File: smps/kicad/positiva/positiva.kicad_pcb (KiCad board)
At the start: 2 copper layers, 124.5 x 72.4 mm, 13 parts, among them J1 Conn_01x01_Female, J2 Conn_01x01_Female, J3 Conn_01x01_Female, J4 Conn_01x01_Female, U1 LM2576T-ADJ

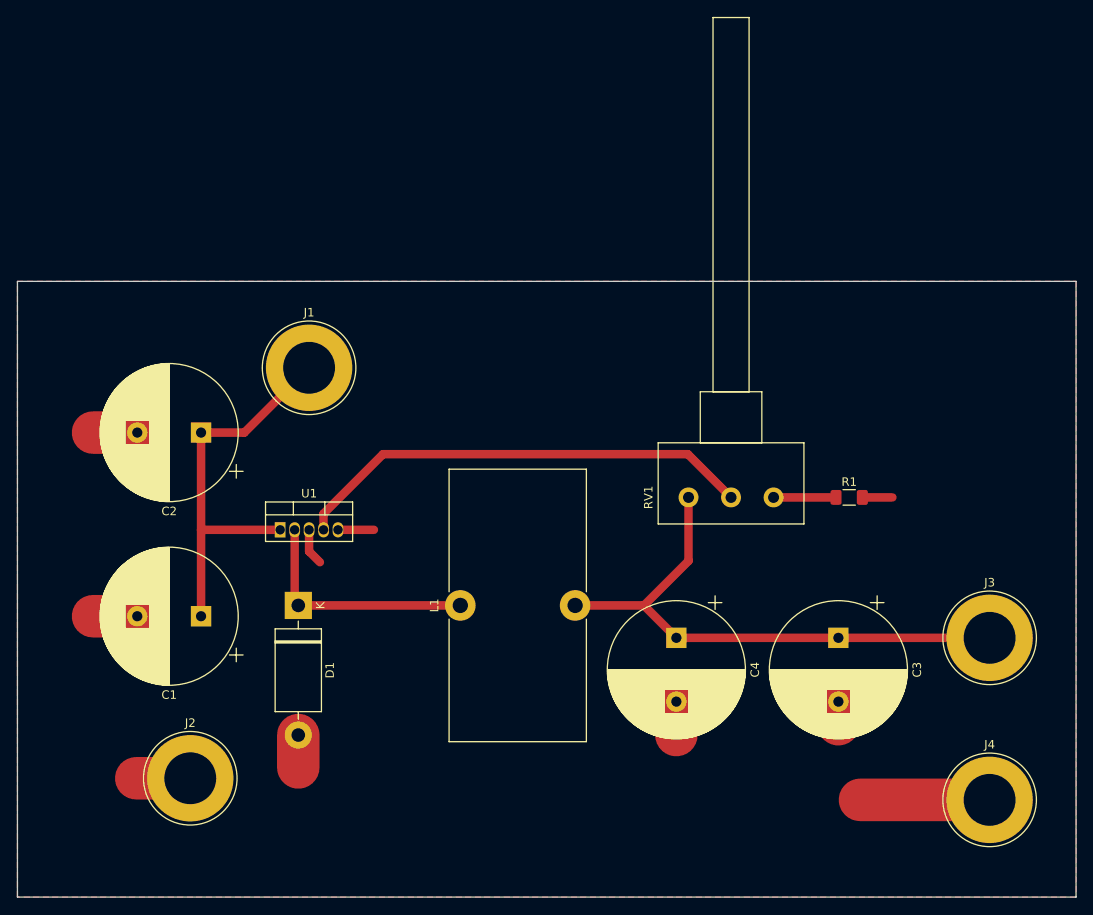
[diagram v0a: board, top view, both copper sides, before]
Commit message: varias cosas, layouts de fuentes terminados, calculo de componentes completo
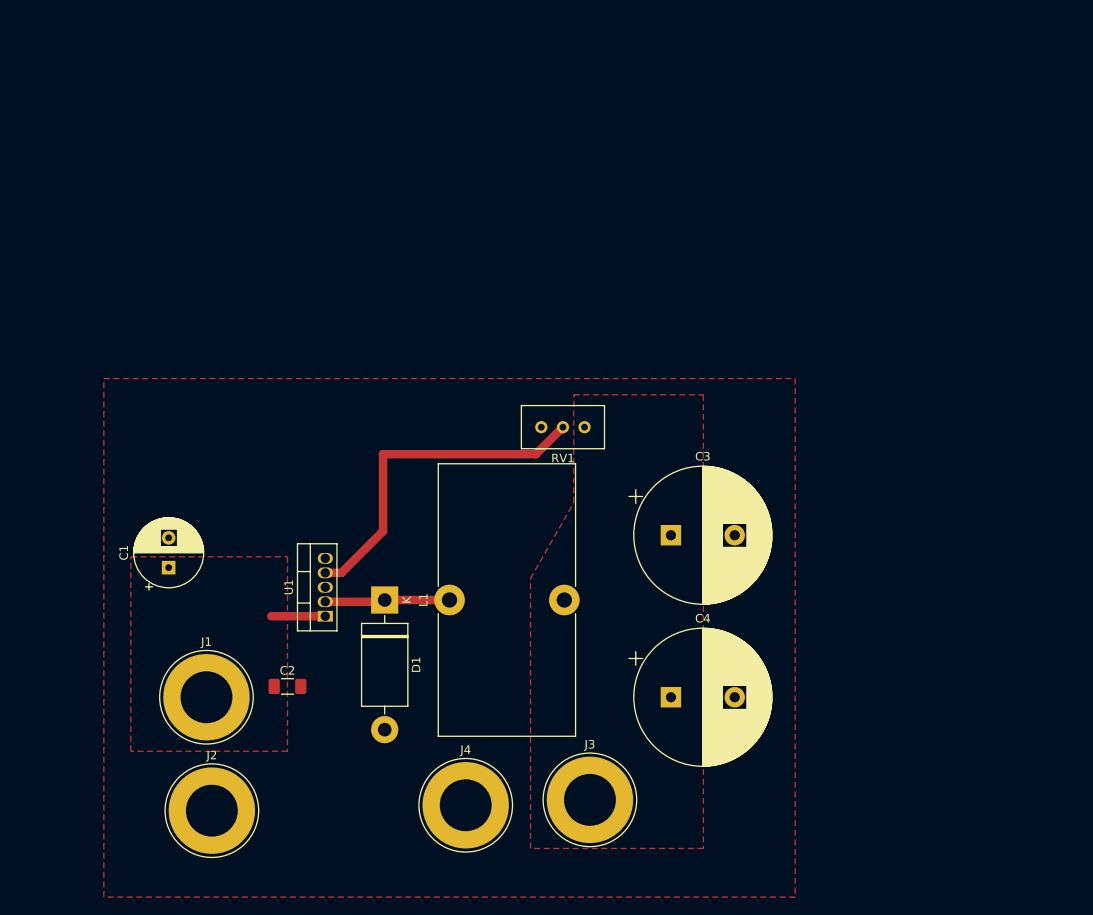
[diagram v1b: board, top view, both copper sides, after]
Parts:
- removed R1: 1.2k, Resistor_SMD:R_1206_3216Metric_Pad1.30x1.75mm_HandSolder
- C1: footprint Capacitor_THT:CP_Radial_D16.0mm_P7.50mm -> Capacitor_THT:CP_Radial_D8.0mm_P3.50mm
- C2: value 100u -> 0.22u; footprint Capacitor_THT:CP_Radial_D16.0mm_P7.50mm -> Capacitor_SMD:C_1206_3216Metric_Pad1.33x1.80mm_HandSolder
- RV1: value 50k -> 100k; footprint Potentiometer_THT:Potentiometer_Omeg_PC16BU_Horizontal -> Potentiometer_THT:Potentiometer_Bourns_3296W_Vertical
- moved J4 61.6 mm to (155.6, 153.0)
- moved J3 50.7 mm to (170.2, 152.4)
- moved J1 40.6 mm to (125.1, 140.3)
- moved C2 31.5 mm to (134.6, 139.1), turned to 0 degrees
- moved RV1 28.5 mm to (164.5, 108.6), turned to 180 degrees
- moved C3 23.1 mm to (179.7, 121.3), turned to 0 degrees
- moved U1 11.5 mm to (139.1, 130.8), turned to 90 degrees
- moved D1 10.2 mm to (146.1, 128.9)
- moved C4 7.01 mm to (179.7, 140.3), turned to 0 degrees
- moved C1 6.87 mm to (120.7, 125.1), turned to 90 degrees
- moved J2 4.58 mm to (125.7, 153.7)
- moved L1 1.42 mm to (153.7, 128.9)
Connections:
- RV1 pad 1: Net-(R1-Pad1) -> GND
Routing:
- net /VoutDC: track 65.2 -> 0.00 mm
- net GND: track 54.5 -> 0.00 mm
- net /Vin: track 46.7 -> 6.35 mm
- net /Vfb: track 54.8 -> 40.3 mm
- net /VoutSW: track 28.7 -> 14.7 mm
- net Net-(R1-Pad1): track 7.34 -> 0.00 mm
- added copper zone on F.Cu, net /Vin
- added copper zone on F.Cu, net /VoutDC
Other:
- board outline removed

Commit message: last minute commit
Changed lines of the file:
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@@
   (general
     (thickness 1.6)
-    (drawings 2)
+    (drawings 0)
     (tracks 9)
     (zones 0)
@@
   )
   (setup
-    (last_trace_width 1)
+    (last_trace_width 0.3048)
     (user_trace_width 1)
     (user_trace_width 5)
@@
     (visible_elements FFFFFF7F)
     (pcbplotparams
-      (layerselection 0x010fc_ffffffff)
+      (layerselection 0x01088_7fffffff)
       (usegerberextensions false)
       (usegerberattributes true)
@@
       (outputformat 1)
       (mirror false)
-      (drillshape 1)
+      (drillshape 0)
       (scaleselection 1)
       (outputdirectory ""))
@@
       (effects (font (size 1 1) (thickness 0.15)))
     )
-    (fp_text user %R (at 0 0) (layer F.Fab)
-      (effects (font (size 0.8 0.8) (thickness 0.12)))
-    )
     (fp_line (start -1.6 0.8) (end -1.6 -0.8) (layer F.Fab) (width 0.1))
     (fp_line (start -1.6 -0.8) (end 1.6 -0.8) (layer F.Fab) (width 0.1))
@@
     (fp_line (start 2.48 -1.15) (end 2.48 1.15) (layer F.CrtYd) (width 0.05))
     (fp_line (start 2.48 1.15) (end -2.48 1.15) (layer F.CrtYd) (width 0.05))
-    (pad 2 smd roundrect (at 1.5625 0) (size 1.325 1.8) (layers F.Cu F.Paste F.Mask) (roundrect_rratio 0.188679)
+    (fp_text user %R (at 0 0) (layer F.Fab)
+      (effects (font (size 0.8 0.8) (thickness 0.12)))
+    )
+    (pad 2 smd roundrect (at 1.5625 0) (size 1.325 1.8) (layers F.Cu F.Paste F.Mask) (roundrect_rratio 0.1886784905660377)
       (net 1 GND))
-    (pad 1 smd roundrect (at -1.5625 0) (size 1.325 1.8) (layers F.Cu F.Paste F.Mask) (roundrect_rratio 0.188679)
+    (pad 1 smd roundrect (at -1.5625 0) (size 1.325 1.8) (layers F.Cu F.Paste F.Mask) (roundrect_rratio 0.1886784905660377)
       (net 2 /Vin))
     (model ${KISYS3DMOD}/Capacitor_SMD.3dshapes/C_1206_3216Metric.wrl
@@
     )
   )
-  (dimension 60.96 (width 0.15) (layer Dwgs.User)
-    (gr_text "60,960 mm" (at 86.33 133.35 90) (layer Dwgs.User)
-      (effects (font (size 1 1) (thickness 0.15)))
-    )
-    (feature1 (pts (xy 113.03 102.87) (xy 87.043579 102.87)))
-    (feature2 (pts (xy 113.03 163.83) (xy 87.043579 163.83)))
-    (crossbar (pts (xy 87.63 163.83) (xy 87.63 102.87)))
-    (arrow1a (pts (xy 87.63 102.87) (xy 88.216421 103.996504)))
-    (arrow1b (pts (xy 87.63 102.87) (xy 87.043579 103.996504)))
-    (arrow2a (pts (xy 87.63 163.83) (xy 88.216421 162.703496)))
-    (arrow2b (pts (xy 87.63 163.83) (xy 87.043579 162.703496)))
-  )
-  (dimension 81.28 (width 0.15) (layer Dwgs.User)
-    (gr_text "81,280 mm" (at 153.67 174.655) (layer Dwgs.User)
-      (effects (font (size 1 1) (thickness 0.15)))
-    )
-    (feature1 (pts (xy 194.31 163.83) (xy 194.31 173.941421)))
-    (feature2 (pts (xy 113.03 163.83) (xy 113.03 173.941421)))
-    (crossbar (pts (xy 113.03 173.355) (xy 194.31 173.355)))
-    (arrow1a (pts (xy 194.31 173.355) (xy 193.183496 173.941421)))
-    (arrow1b (pts (xy 194.31 173.355) (xy 193.183496 172.768579)))
-    (arrow2a (pts (xy 113.03 173.355) (xy 114.156504 173.941421)))
-    (arrow2b (pts (xy 113.03 173.355) (xy 114.156504 172.768579)))
-  )
   (segment (start 139.065 130.81) (end 132.715 130.81) (width 1) (layer F.Cu) (net 2))
   (segment (start 145.845 129.11) (end 146.05 128.905) (width 1) (layer F.Cu) (net 4))
@@
   (zone (net 2) (net_name /Vin) (layer F.Cu) (hatch edge 0.508)
     (priority 1)
-    (connect_pads (clearance 1))
+    (connect_pads yes (clearance 1))
     (min_thickness 0.254)
     (fill yes (arc_segments 32) (thermal_gap 0.508) (thermal_bridge_width 0.508))
